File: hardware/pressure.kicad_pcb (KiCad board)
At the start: 2 copper layers, 17.5 x 25 mm, 19 parts, among them P1 CON-SENSOR, Q1 2N7002P, U1 M24C64, U2 DRILL, U3 DRILL, U4 DRILL, U5 DRILL

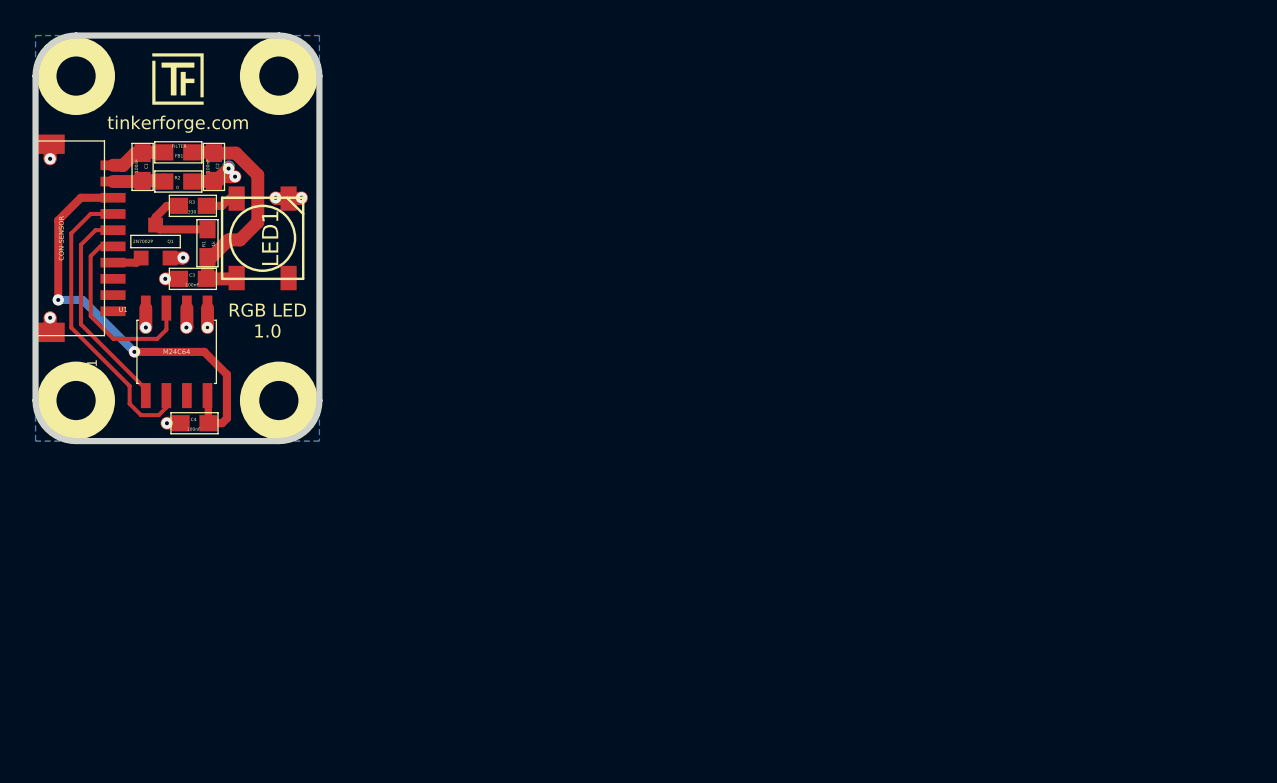
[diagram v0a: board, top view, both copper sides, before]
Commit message: pressure bricklet hardware prototype
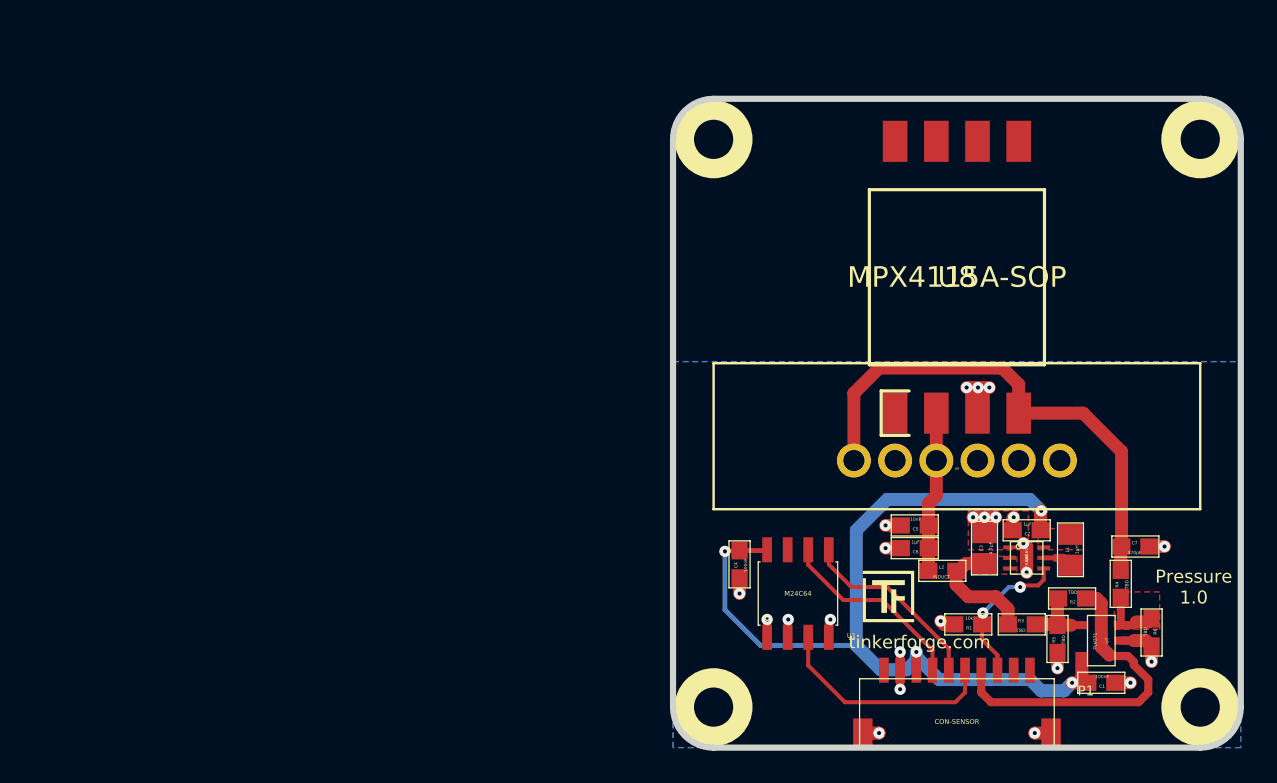
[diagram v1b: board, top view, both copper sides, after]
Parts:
- removed FB1: FILTER, kicad-libraries:0603E
- removed LED1: WS2812B_LED, kicad-libraries:WS2812B_LED
- removed Q1: 2N7002P, kicad-libraries:SOT23GDS
- added C5: 10nF, kicad-libraries:0603E, F.Cu at (179.5, 135.8)
- added C6: 1µF, kicad-libraries:0603E, F.Cu at (179.5, 137.2)
- added C7: 470pF, kicad-libraries:0603E, F.Cu at (193.1, 137.1)
- added L1: 1µH, kicad-libraries:0805E, F.Cu at (189.1, 137.3)
- added L2: INDUCT, kicad-libraries:0603E, F.Cu at (181.2, 138.6)
- added R4: TBD, kicad-libraries:0603E, F.Cu at (192.2, 139.4)
- added R5: TBD, kicad-libraries:0603E, F.Cu at (188.3, 142.8)
- added R6: TBD, kicad-libraries:0603E, F.Cu at (194.1, 142.4)
- added U6: FAN4860, kicad-libraries:UMLP_22, F.Cu at (186.4, 137.8)
- added U7: TLV271, kicad-libraries:SOT23-5, F.Cu at (191.0, 142.9)
- added U8: MPX4115A-SOP, kicad-libraries:SOP8, F.Cu at (182.1, 120.5)
- added U9: MPX_UNI, kicad-libraries:MPX_UNI, F.Cu at (182.1, 131.8)
- C2: value 100nF -> 1µF
- C3: value 100nF -> 4.7µF; footprint kicad-libraries:0603E -> kicad-libraries:0805E
- R1: value 1k -> 10k
- R2: value 0 -> TBD
- R3: value 330 -> TBD
- moved C1 67.1 mm to (191.0, 145.5), turned to 0 degrees
- moved P1 64.9 mm to (182.1, 149.5), turned to 0 degrees
- moved R2 60.8 mm to (189.2, 140.3), turned to 0 degrees
- moved U3 59.9 mm to (197.1, 147.0)
- moved R3 57.2 mm to (186.1, 141.9)
- moved U5 56.9 mm to (197.1, 112.0)
- moved C2 54.9 mm to (186.4, 136.1), turned to 0 degrees
- moved G*** 54.2 mm to (176.3, 138.6)
- moved VAL 53.2 mm to (189.8, 126.8)
- moved R1 52.5 mm to (182.8, 141.9), turned to 0 degrees
- moved C3 51.5 mm to (183.8, 137.2), turned to 270 degrees
- moved G*** 44.9 mm to (174.4, 126.8)
- moved U4 43.6 mm to (167.1, 147.0)
- moved U1 41.1 mm to (172.3, 140.0), turned to 0 degrees
- moved U2 39.5 mm to (167.1, 112.0)
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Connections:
- C1 pad 1: Net-(C1-Pad1) -> 3V3
- C1 pad 2: Net-(C1-Pad2) -> GND
- C2 pad 2: VCC -> 3V3
- C3 pad 1: VCC -> GND
- C3 pad 2: GND -> +5V
- P1 pad 1: Net-(C1-Pad2) -> (no net)
- P1 pad 2: Net-(C1-Pad1) -> GND
- P1 pad 8: (no net) -> Net-(P1-Pad8)
- R1 pad 1: Net-(Q1-PadD) -> GND
- R1 pad 2: VCC -> Net-(P1-Pad8)
- R2 pad 1: GND -> Net-(R2-Pad1)
- R2 pad 2: Net-(C1-Pad1) -> Net-(P1-Pad7)
- R3 pad 1: Net-(LED1-Pad4) -> Net-(R2-Pad1)
- R3 pad 2: Net-(Q1-PadD) -> +5V
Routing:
- net Net-(C7-Pad2): track 0.00 -> 31.8 mm
- net 3V3: track 26.9 -> 56.0 mm, vias 2 -> 4
- net Net-(P1-Pad7): track 1.85 -> 20.6 mm
- net VCC: track 14.8 -> 0.00 mm
- net GND: track 13.6 -> 27.5 mm, vias 12 -> 24
- net Net-(C5-Pad2): track 0.00 -> 9.92 mm
- net Net-(P1-Pad8): track 0.00 -> 9.24 mm, vias 0 -> 2
- net +5V: track 0.00 -> 7.56 mm
- net SCL: track 18.6 -> 12.0 mm
- net Net-(Q1-PadD): track 5.53 -> 0.00 mm
- net Net-(R2-Pad1): track 0.00 -> 4.61 mm
- net Net-(R4-Pad2): track 0.00 -> 3.84 mm
- net Net-(C1-Pad2): track 3.51 -> 0.00 mm
- net Net-(C1-Pad1): track 3.29 -> 0.00 mm
- net Net-(LED1-Pad4): track 2.04 -> 0.00 mm
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- added copper zone on F.Cu, net +5V
- added copper zone on F.Cu, net 3V3
- added copper zone on F.Cu, net GND
- added copper zone on F.Cu, net Net-(R4-Pad2)
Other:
- board size 17.5 x 25 mm -> 35 x 40 mm
- board text added: "Pressure 1.0"
- board text removed: "RGB LED 1.0"
